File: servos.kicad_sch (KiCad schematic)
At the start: 12 parts, among them J10 171857-0003, J11 171857-0003, J12 171857-0003, J13 171857-0003

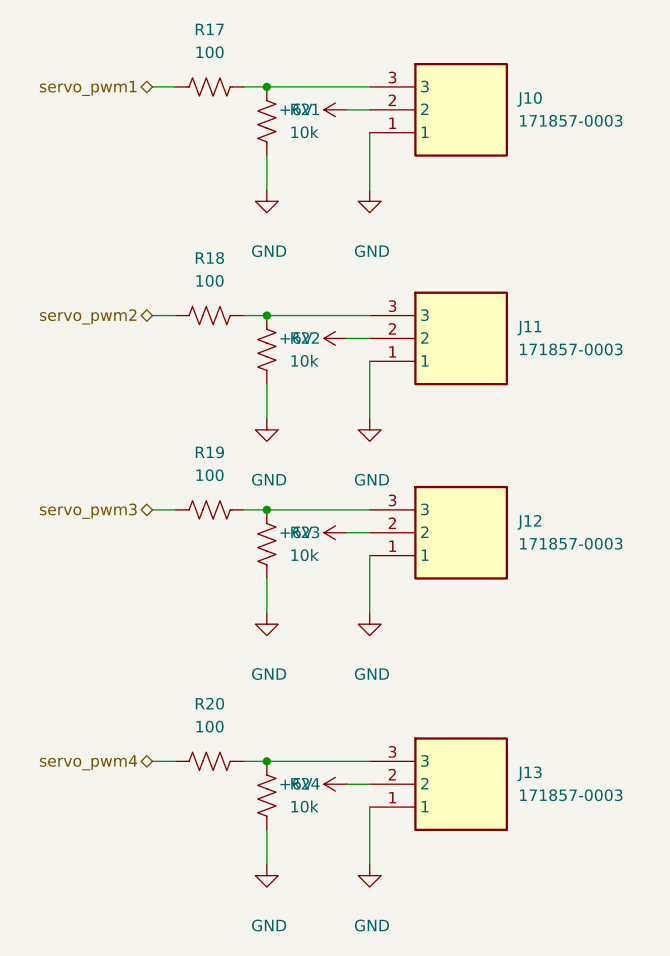
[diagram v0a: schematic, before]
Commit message: feat: final changes, sent to prod
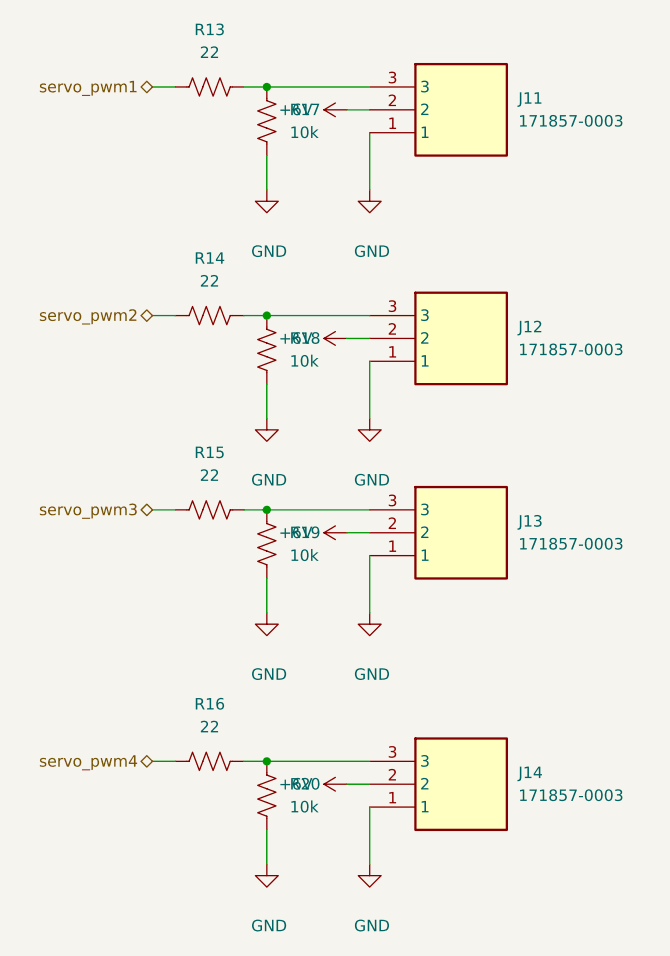
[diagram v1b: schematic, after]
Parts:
- R13: renamed from R17; value 100 -> 22
- R14: renamed from R18; value 100 -> 22
- R15: renamed from R19; value 100 -> 22
- R16: renamed from R20; value 100 -> 22
- renumbered J10 to J11, J11 to J12, J12 to J13, J13 to J14, R21 to R17, R22 to R18, R23 to R19, R24 to R20

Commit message: Revised componenents, need to route
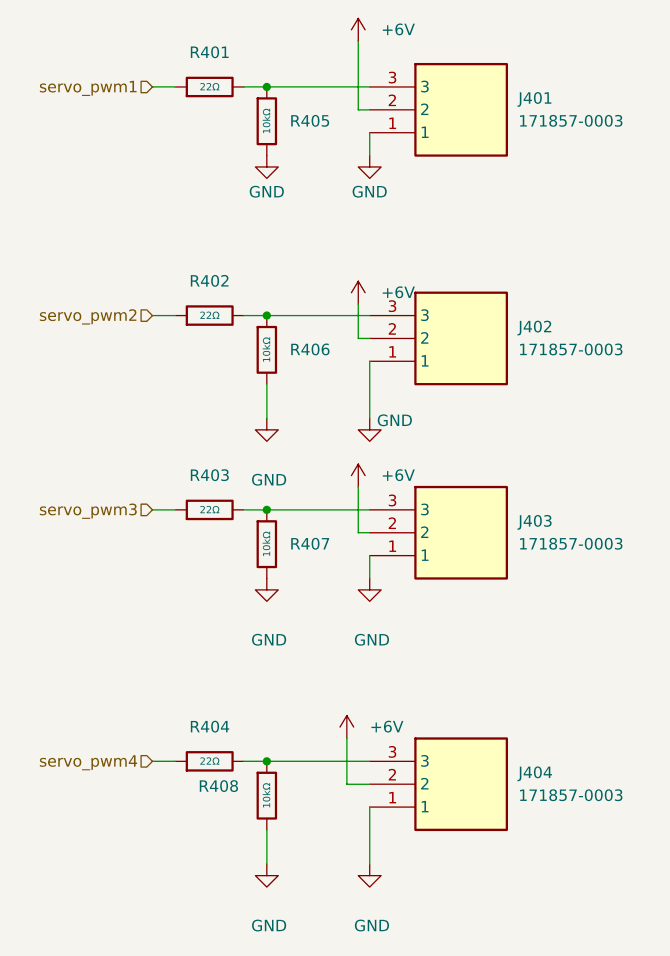
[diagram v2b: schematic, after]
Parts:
- removed R13, R14, R15, R16: 22, PCM_SparkFun-Resistor:R_0603_1608Metric, symbol PCM_SparkFun-Resistor:R
- removed R17, R18, R19, R20: 10k, PCM_SparkFun-Resistor:R_0603_1608Metric, symbol PCM_SparkFun-Resistor:R
- added R401, R402, R403, R404: 22Ω, PCM_JLCPCB:R_0402, symbol PCM_JLCPCB-Resistors:0402,22Ω
- added R405, R406, R407, R408: 10kΩ, PCM_JLCPCB:R_0402, symbol PCM_JLCPCB-Resistors:0402,10kΩ
- renumbered J11 to J401, J12 to J402, J13 to J403, J14 to J404
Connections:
- net GND: now also R405.2, R406.2, R407.2, R408.2
- net servo_pwm1: now also R401.1
- net servo_pwm2: now also R402.1
- net servo_pwm3: now also R403.1
- net servo_pwm4: now also R404.1
- net at J404.3: now also R404.2, R408.1
- net at J403.3: now also R403.2, R407.1
- net at J401.3: now also R401.2, R405.1
- net at J402.3: now also R402.2, R406.1
